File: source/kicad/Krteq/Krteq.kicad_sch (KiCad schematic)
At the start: 202 parts, among them J1 USB breakout board, J2 Pico test points, J3 OLED 128x32, SW1 GATERON Low Profile Switch Ho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, SW10 GATERON Low Profile Switch Ho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, SW11 GATERON Low Profile Switch Ho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, SW12 GATERON Low Profile Switch Ho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, SW13 GATERON Low Profile Switch Ho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, SW14 GATERON Low Profile Switch Ho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, SW15 GATERON Low Profile Switch Ho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, SW16 GATERON Low Profile Switch Ho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, SW17 GATERON Low Profile Switch Ho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, SW18 GATERON Low Profile Switch Ho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, SW19 GATERON Low Profile Switch Ho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, SW2 GATERON Low Profile Switch Ho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, SW20 GATERON Low Profile Switch Ho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, SW21 GATERON Low Profile Switch Ho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, SW22 GATERON Low Profile Switch Ho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, SW23 GATERON Low Profile Switch Ho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, SW24 GATERON Low Profile Switch Ho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, SW25 GATERON Low Profile Switch Ho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, SW26 GATERON Low Profile Switch Ho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, SW27 GATERON Low Profile Switch Ho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, SW28 GATERON Low Profile Switch Ho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, SW29 GATERON Low Profile Switch Ho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, SW3 GATERON Low Profile Switch Ho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, SW30 GATERON Low Profile Switch Ho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, SW31 GATERON Low Profile Switch Ho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, SW32 GATERON Low Profile Switch Ho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, SW33 GATERON Low Profile Switch Ho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, SW34 GATERON Low Profile Switch Ho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, SW35 GATERON Low Profile Switch Ho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, SW36 GATERON Low Profile Switch Ho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, SW37 GATERON Low Profile Switch Ho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, SW38 GATERON Low Profile Switch Ho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, SW39 GATERON Low Profile Switch Ho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, SW4 GATERON Low Profile Switch Ho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, SW40 GATERON Low Profile Switch Ho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, SW41 GATERON Low Profile Switch Ho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, SW42 GATERON Low Profile Switch Ho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, SW43 GATERON Low Profile Switch Ho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, SW44 GATERON Low Profile Switch Ho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, SW45 GATERON Low Profile Switch Ho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, SW46 GATERON Low Profile Switch Ho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, SW47 GATERON Low Profile Switch Ho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, SW48 GATERON Low Profile Switch Ho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, SW49 GATERON Low Profile Switch Ho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, SW5 GATERON Low Profile Switch Ho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, SW50 GATERON Low Profile Switch Ho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, SW51 GATERON Low Profile Switch Ho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, SW52 GATERON Low Profile Switch Ho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, SW53 GATERON Low Profile Switch Ho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, SW54 GATERON Low Profile Switch Ho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, SW55 GATERON Low Profile Switch Ho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, SW56 GATERON Low Profile Switch Ho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, SW57 GATERON Low Profile Switch Ho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, SW58 GATERON Low Profile Switch Ho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, SW59 GATERON Low Profile Switch Ho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, SW6 GATERON Low Profile Switch Ho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, SW60 GATERON Low Profile Switch Ho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, SW61 GATERON Low Profile Switch Ho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, SW7 GATERON Low Profile Switch Ho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, SW8 GATERON Low Profile Switch Ho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, SW9 GATERON Low Profile Switch Ho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, U71 IS31FL3733-QF

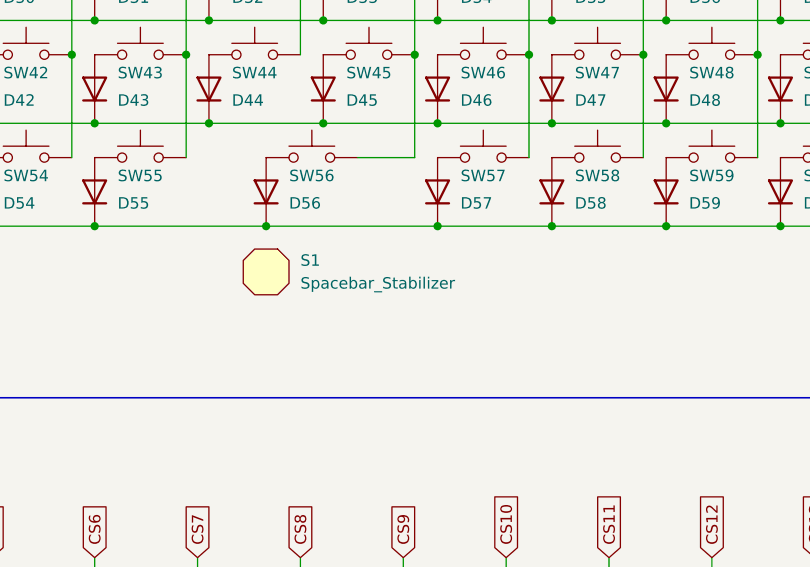
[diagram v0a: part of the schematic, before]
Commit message: bom update
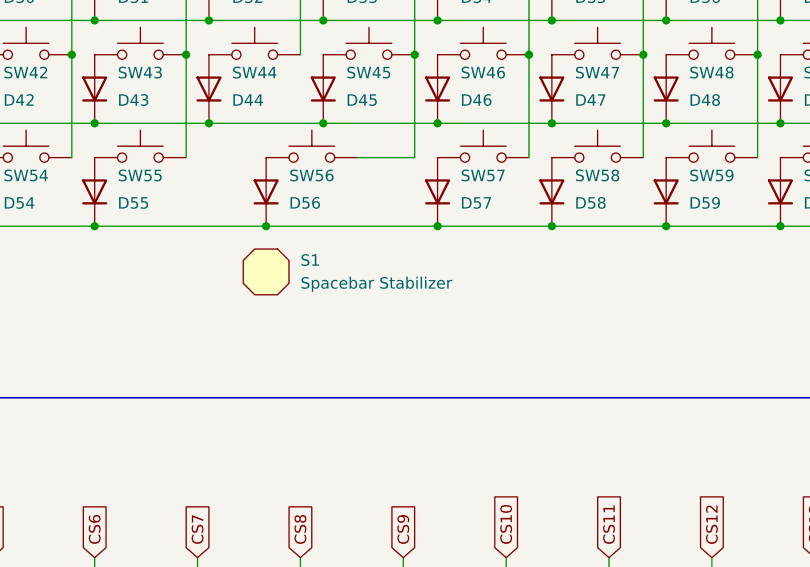
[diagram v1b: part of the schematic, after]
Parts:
- D101, D102, D103, D104, D105, D106, D107, D108, D109, D110, D111, D112, D113, D114, D115, D116, D117, D118, D119, D120, D121, D122, D123, D124, D125, D126, D127, D128, D129, D130, D131, D132, D133, D134, D135, D136, D137, D138, D139, D140, D141, D142, D143, D144, D145, D146, D147, D148, D149, D150, D151, D152, D153, D154, D155, D156, D157, D158, D159, D160, D161: value LED_ABGR -> Reverse Mount LED ABGR
- S1: value Spacebar_Stabilizer -> Spacebar Stabilizer
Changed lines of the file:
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@@
 			)
 		)
-		(property "Value" "LED_ABGR"
+		(property "Value" "Reverse Mount LED ABGR"
 			(at 184.15 208.28 0)
 			(hide yes)
@@
 			)
 		)
-		(property "Value" "LED_ABGR"
+		(property "Value" "Reverse Mount LED ABGR"
 			(at 218.44 209.55 0)
 			(hide yes)
@@
 			)
 		)
-		(property "Value" "LED_ABGR"
+		(property "Value" "Reverse Mount LED ABGR"
 			(at 218.44 189.23 0)
 			(hide yes)
@@
 			)
 		)
-		(property "Value" "LED_ABGR"
+		(property "Value" "Reverse Mount LED ABGR"
 			(at 229.87 167.64 0)
 			(hide yes)
@@
 			)
 		)
-		(property "Value" "LED_ABGR"
+		(property "Value" "Reverse Mount LED ABGR"
 			(at 275.59 208.28 0)
 			(hide yes)
@@
 			)
 		)
-		(property "Value" "LED_ABGR"
+		(property "Value" "Reverse Mount LED ABGR"
 			(at 229.87 187.96 0)
 			(hide yes)
@@
 			)
 		)
-		(property "Value" "LED_ABGR"
+		(property "Value" "Reverse Mount LED ABGR"
 			(at 298.45 167.64 0)
 			(hide yes)
@@
 			)
 		)
-		(property "Value" "LED_ABGR"
+		(property "Value" "Reverse Mount LED ABGR"
 			(at 195.58 148.59 0)
 			(hide yes)
@@
 			)
 		)
-		(property "Value" "LED_ABGR"
+		(property "Value" "Reverse Mount LED ABGR"
 			(at 264.16 209.55 0)
 			(hide yes)
@@
 			)
 		)
-		(property "Value" "LED_ABGR"
+		(property "Value" "Reverse Mount LED ABGR"
 			(at 264.16 168.91 0)
 			(hide yes)
@@
 			)
 		)
-		(property "Value" "LED_ABGR"
+		(property "Value" "Reverse Mount LED ABGR"
 			(at 321.31 187.96 0)
 			(hide yes)
@@
 			)
 		)
-		(property "Value" "LED_ABGR"
+		(property "Value" "Reverse Mount LED ABGR"
 			(at 344.17 187.96 0)
 			(hide yes)
@@
 			)
 		)
-		(property "Value" "LED_ABGR"
+		(property "Value" "Reverse Mount LED ABGR"
 			(at 207.01 187.96 0)
 			(hide yes)
@@
 			)
 		)
-		(property "Value" "LED_ABGR"
+		(property "Value" "Reverse Mount LED ABGR"
 			(at 207.01 147.32 0)
 			(hide yes)
@@
 			)
 		)
-		(property "Value" "LED_ABGR"
+		(property "Value" "Reverse Mount LED ABGR"
 			(at 275.59 187.96 0)
 			(hide yes)
@@
 			)
 		)
-		(property "Value" "LED_ABGR"
+		(property "Value" "Reverse Mount LED ABGR"
 			(at 241.3 189.23 0)
 			(hide yes)
@@
 			)
 		)
-		(property "Value" "Spacebar_Stabilizer"
+		(property "Value" "Spacebar Stabilizer"
 			(at 257.81 113.0299 0)
 			(show_name no)
@@
 			)
 		)
-		(property "Value" "LED_ABGR"
+		(property "Value" "Reverse Mount LED ABGR"
 			(at 332.74 209.55 0)
 			(hide yes)
@@
 			)
 		)
-		(property "Value" "LED_ABGR"
+		(property "Value" "Reverse Mount LED ABGR"
 			(at 321.31 147.32 0)
 			(hide yes)
@@
 			)
 		)
-		(property "Value" "LED_ABGR"
+		(property "Value" "Reverse Mount LED ABGR"
 			(at 252.73 208.28 0)
 			(hide yes)
@@
 			)
 		)
-		(property "Value" "LED_ABGR"
+		(property "Value" "Reverse Mount LED ABGR"
 			(at 207.01 167.64 0)
 			(hide yes)
@@
 			)
 		)
-		(property "Value" "LED_ABGR"
+		(property "Value" "Reverse Mount LED ABGR"
 			(at 298.45 147.32 0)
 			(hide yes)
@@
 			)
 		)
-		(property "Value" "LED_ABGR"
+		(property "Value" "Reverse Mount LED ABGR"
 			(at 309.88 148.59 0)
 			(hide yes)
@@
 			)
 		)
-		(property "Value" "LED_ABGR"
+		(property "Value" "Reverse Mount LED ABGR"
 			(at 252.73 167.64 0)
 			(hide yes)
@@
 			)
 		)
-		(property "Value" "LED_ABGR"
+		(property "Value" "Reverse Mount LED ABGR"
 			(at 287.02 168.91 0)
 			(hide yes)
@@
 			)
 		)
-		(property "Value" "LED_ABGR"
+		(property "Value" "Reverse Mount LED ABGR"
 			(at 229.87 208.28 0)
 			(hide yes)
@@
 			)
 		)
-		(property "Value" "LED_ABGR"
+		(property "Value" "Reverse Mount LED ABGR"
 			(at 241.3 209.55 0)
 			(hide yes)
@@
 			)
 		)
-		(property "Value" "LED_ABGR"
+		(property "Value" "Reverse Mount LED ABGR"
 			(at 287.02 209.55 0)
 			(hide yes)
@@
 			)
 		)
-		(property "Value" "LED_ABGR"
+		(property "Value" "Reverse Mount LED ABGR"
 			(at 252.73 187.96 0)
 			(hide yes)
@@
 			)
 		)
-		(property "Value" "LED_ABGR"
+		(property "Value" "Reverse Mount LED ABGR"
 			(at 252.73 147.32 0)
 			(hide yes)
@@
 			)
 		)
-		(property "Value" "LED_ABGR"
+		(property "Value" "Reverse Mount LED ABGR"
 			(at 241.3 148.59 0)
 			(hide yes)
@@
 			)
 		)
-		(property "Value" "LED_ABGR"
+		(property "Value" "Reverse Mount LED ABGR"
 			(at 229.87 147.32 0)
 			(hide yes)
@@
 			)
 		)
-		(property "Value" "LED_ABGR"
+		(property "Value" "Reverse Mount LED ABGR"
 			(at 321.31 208.28 0)
 			(hide yes)
@@
 			)
 		)
-		(property "Value" "LED_ABGR"
+		(property "Value" "Reverse Mount LED ABGR"
 			(at 184.15 187.96 0)
 			(hide yes)
@@
 			)
 		)
-		(property "Value" "LED_ABGR"
+		(property "Value" "Reverse Mount LED ABGR"
 			(at 195.58 168.91 0)
 			(hide yes)
@@
 			)
 		)
-		(property "Value" "LED_ABGR"
+		(property "Value" "Reverse Mount LED ABGR"
 			(at 344.17 147.32 0)
 			(hide yes)
@@
 			)
 		)
-		(property "Value" "LED_ABGR"
+		(property "Value" "Reverse Mount LED ABGR"
 			(at 218.44 168.91 0)
 			(hide yes)
@@
 			)
 		)
-		(property "Value" "LED_ABGR"
+		(property "Value" "Reverse Mount LED ABGR"
 			(at 264.16 148.59 0)
 			(hide yes)
@@
 			)
 		)
-		(property "Value" "LED_ABGR"
+		(property "Value" "Reverse Mount LED ABGR"
 			(at 321.31 167.64 0)
 			(hide yes)
@@
 			)
 		)
-		(property "Value" "LED_ABGR"
+		(property "Value" "Reverse Mount LED ABGR"
 			(at 298.45 208.28 0)
 			(hide yes)
@@
 			)
 		)
-		(property "Value" "LED_ABGR"
+		(property "Value" "Reverse Mount LED ABGR"
 			(at 195.58 209.55 0)
 			(hide yes)
@@
 			)
 		)
-		(property "Value" "LED_ABGR"
+		(property "Value" "Reverse Mount LED ABGR"
 			(at 172.72 148.59 0)
 			(hide yes)
@@
 			)
 		)
-		(property "Value" "LED_ABGR"
+		(property "Value" "Reverse Mount LED ABGR"
 			(at 344.17 208.28 0)
 			(hide yes)
@@
 			)
 		)
-		(property "Value" "LED_ABGR"
+		(property "Value" "Reverse Mount LED ABGR"
 			(at 287.02 189.23 0)
 			(hide yes)
@@
 			)
 		)
-		(property "Value" "LED_ABGR"
+		(property "Value" "Reverse Mount LED ABGR"
 			(at 195.58 189.23 0)
 			(hide yes)
@@
 			)
 		)
-		(property "Value" "LED_ABGR"
+		(property "Value" "Reverse Mount LED ABGR"
 			(at 332.74 189.23 0)
 			(hide yes)
@@
 			)
 		)
-		(property "Value" "LED_ABGR"
+		(property "Value" "Reverse Mount LED ABGR"
 			(at 184.15 167.64 0)
 			(hide yes)
@@
 			)
 		)
-		(property "Value" "LED_ABGR"
+		(property "Value" "Reverse Mount LED ABGR"
 			(at 344.17 167.64 0)
 			(hide yes)
@@
 			)
 		)
-		(property "Value" "LED_ABGR"
+		(property "Value" "Reverse Mount LED ABGR"
 			(at 287.02 148.59 0)
 			(hide yes)
@@
 			)
 		)
-		(property "Value" "LED_ABGR"
+		(property "Value" "Reverse Mount LED ABGR"
 			(at 241.3 168.91 0)
 			(hide yes)
@@
 			)
 		)
-		(property "Value" "LED_ABGR"
+		(property "Value" "Reverse Mount LED ABGR"
 			(at 264.16 189.23 0)
 			(hide yes)
@@
 			)
 		)
-		(property "Value" "LED_ABGR"
+		(property "Value" "Reverse Mount LED ABGR"
 			(at 172.72 209.55 0)
 			(hide yes)
@@
 			)
 		)
-		(property "Value" "LED_ABGR"
+		(property "Value" "Reverse Mount LED ABGR"
 			(at 207.01 208.28 0)
 			(hide yes)
@@
 			)
 		)
-		(property "Value" "LED_ABGR"
+		(property "Value" "Reverse Mount LED ABGR"
 			(at 309.88 189.23 0)
 			(hide yes)
@@
 			)
 		)
-		(property "Value" "LED_ABGR"
+		(property "Value" "Reverse Mount LED ABGR"
 			(at 298.45 187.96 0)
 			(hide yes)
@@
 			)
 		)
-		(property "Value" "LED_ABGR"
+		(property "Value" "Reverse Mount LED ABGR"
 			(at 275.59 147.32 0)
 			(hide yes)
@@
 			)
 		)
-		(property "Value" "LED_ABGR"
+		(property "Value" "Reverse Mount LED ABGR"
 			(at 309.88 209.55 0)
 			(hide yes)
@@
 			)
 		)
-		(property "Value" "LED_ABGR"
+		(property "Value" "Reverse Mount LED ABGR"
 			(at 218.44 148.59 0)
 			(hide yes)
@@
 			)
 		)
-		(property "Value" "LED_ABGR"
+		(property "Value" "Reverse Mount LED ABGR"
 			(at 309.88 168.91 0)
 			(hide yes)
@@
 			)
 		)
-		(property "Value" "LED_ABGR"
+		(property "Value" "Reverse Mount LED ABGR"
 			(at 184.15 147.32 0)
 			(hide yes)
@@
 			)
 		)
-		(property "Value" "LED_ABGR"
+		(property "Value" "Reverse Mount LED ABGR"
 			(at 332.74 148.59 0)
 			(hide yes)
@@
 			)
 		)
-		(property "Value" "LED_ABGR"
+		(property "Value" "Reverse Mount LED ABGR"
 			(at 275.59 167.64 0)
 			(hide yes)

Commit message: update
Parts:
- U71: footprint Package_DFN_QFN:QFN-48-1EP_6x6mm_P0.4mm_EP4.4x4.4mm -> Krteq:QFN-48_6x6mm
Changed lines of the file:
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@@
 			)
 		)
-		(property "Footprint" "Package_DFN_QFN:QFN-48-1EP_6x6mm_P0.4mm_EP4.4x4.4mm"
+		(property "Footprint" "Krteq:QFN-48_6x6mm"
 			(at 86.36 219.71 0)
 			(hide yes)
